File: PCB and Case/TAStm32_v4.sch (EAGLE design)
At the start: 45 parts, among them IC4 74LVC14, IC5 74HCT125, IC7 74LVC07, J1 ZX62D-B-5PA8, J10 RJSSE538002, J11 RJSSE538002, J12 SOICBITE, J13 CONSOLE_RESET, J2 UE27-AC54-100, J3 TSM-105-02-L-SHJ, J4 CONSOLE_RESET, J5 OLED128X64, J6 SAMTEC-TSM-116-01-X-SVJ, J7 SAMTEC-TSM-116-01-X-SVJ, U1 STM32F446RET6, U2 3.3V REG, Y1 8MHz

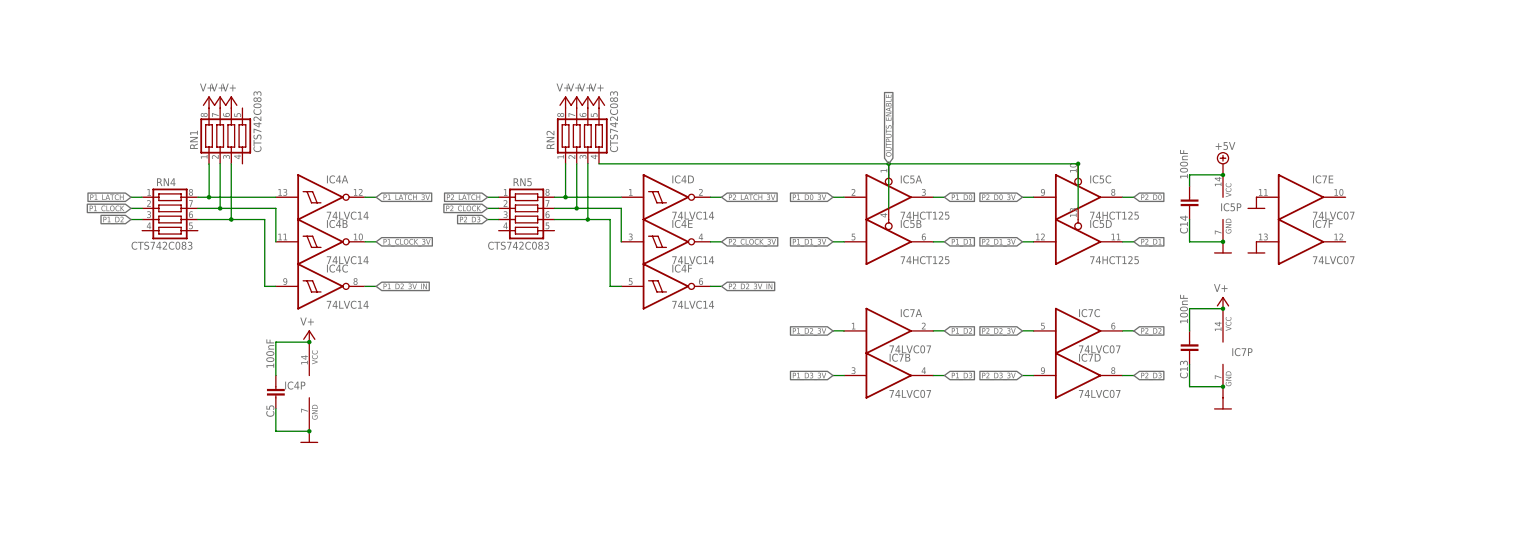
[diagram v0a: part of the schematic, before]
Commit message: caps
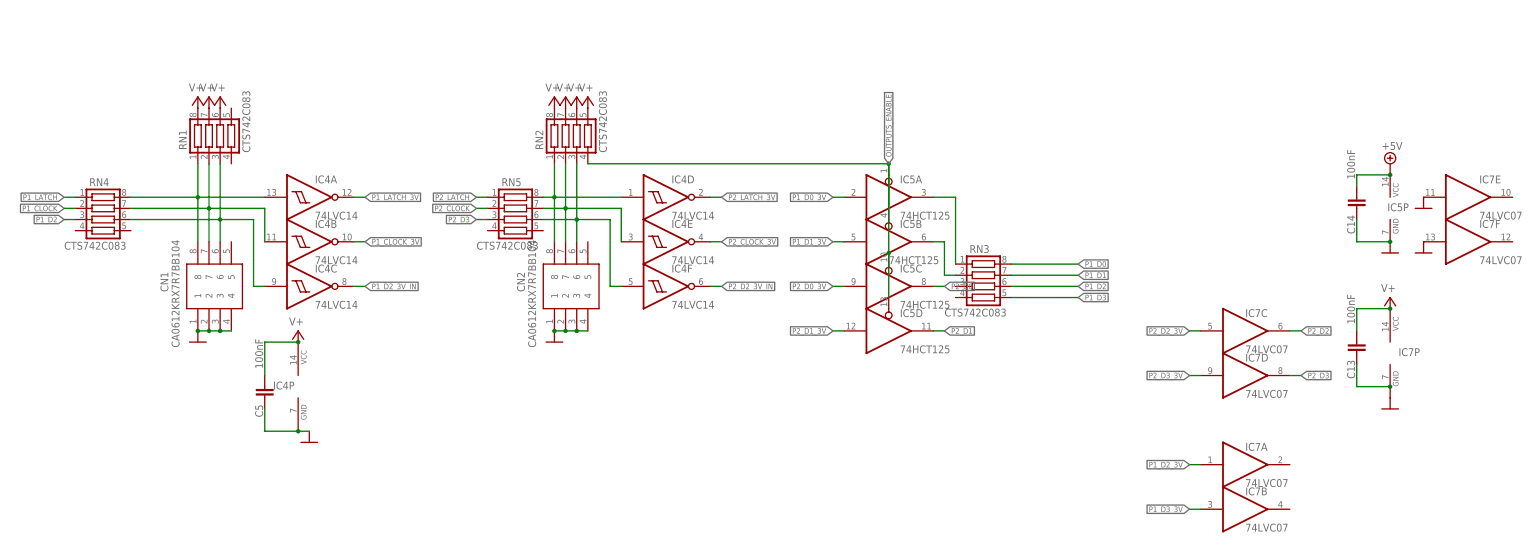
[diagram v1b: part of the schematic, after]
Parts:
- added CN1, CN2: CA0612KRX7R7BB104, SamacSys_Parts:CA0612KRX7R7BB104
- added RN3: CTS742C083, resistor-net:CTS742C083
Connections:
- removed net N$21: IC4F.I, RN2.3, RN5.6
- new net N$4: CN2.8, IC4D.I, RN2.1, RN5.8
- new net N$6: CN2.7, IC4E.I, RN2.2, RN5.7
- new net N$8: CN2.6, IC4F.I, RN2.3, RN5.6
- net GND: now also CN1.1, CN1.2, CN1.3, CN1.4, CN2.1, CN2.2, CN2.3, CN2.4
- net N$16: now also CN1.8
- net N$17: now also CN1.7
- net N$18: now also CN1.6
- net N$2: now also IC5B.O, RN3.2; no longer IC4D.I, RN2.1, RN5.8
- net N$3: now also IC5A.O, RN3.1; no longer IC4E.I, RN2.2, RN5.7
- net P1_D0: now also RN3.8; no longer IC5A.O
- net P1_D1: now also RN3.7; no longer IC5B.O
- net P1_D2: now also RN3.6; no longer IC7A.O
- net P1_D3: now also RN3.5; no longer IC7B.O
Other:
- moved on the sheet: C13, C14, C5, IC4A, IC4B, IC4C, IC4P, IC5C, IC5D, IC5P, IC7A, IC7B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
